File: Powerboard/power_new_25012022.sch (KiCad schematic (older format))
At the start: 25 parts

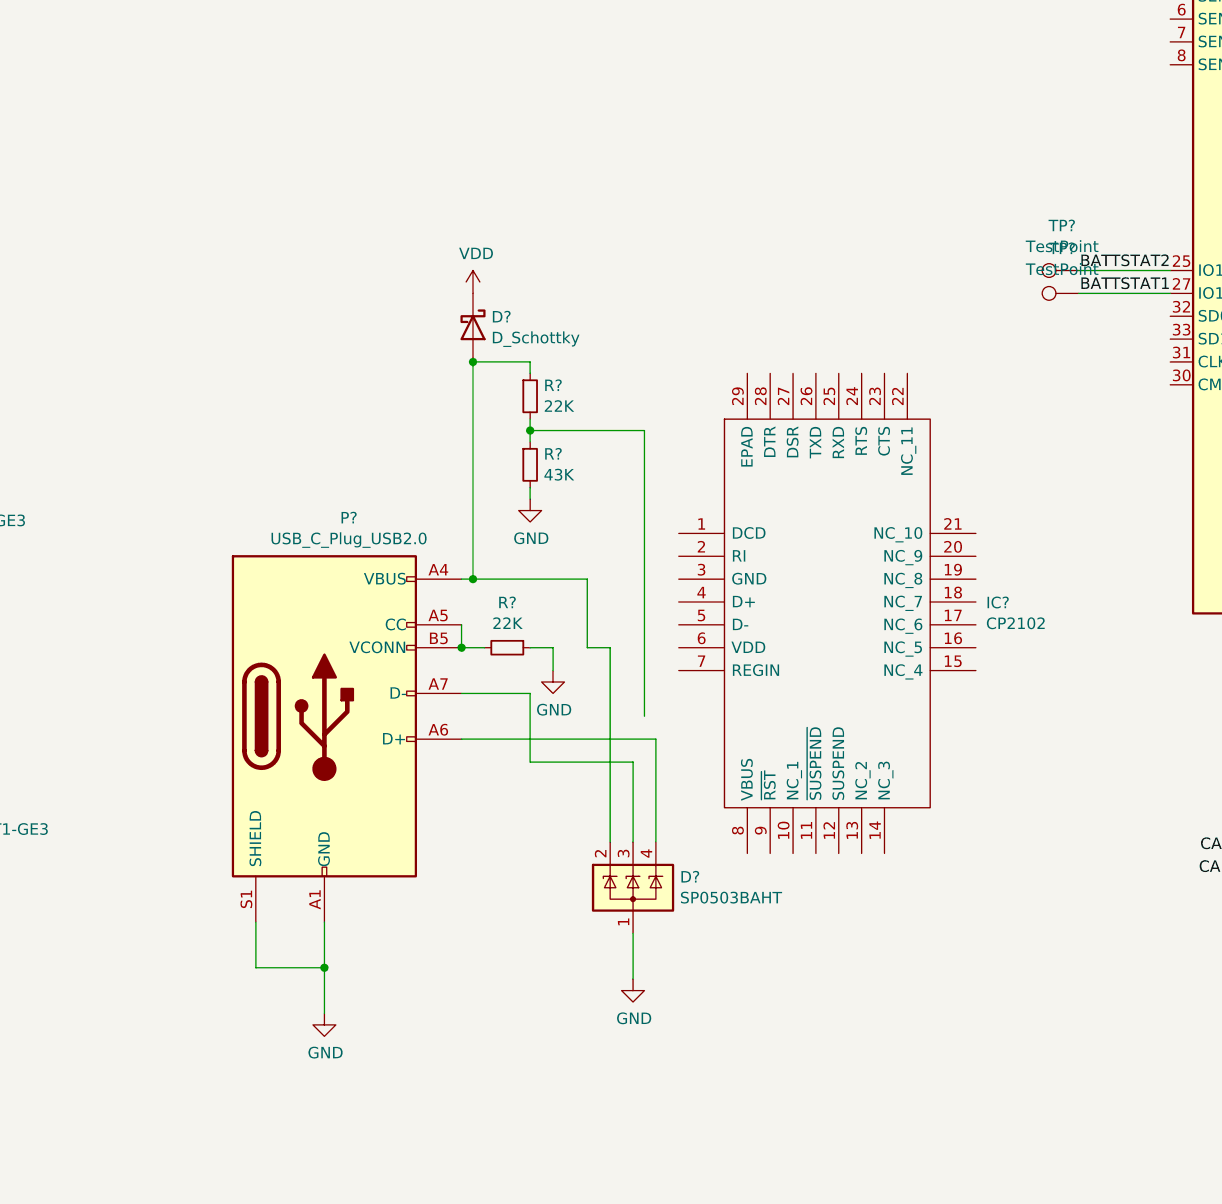
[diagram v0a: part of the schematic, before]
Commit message: 19/02/2022
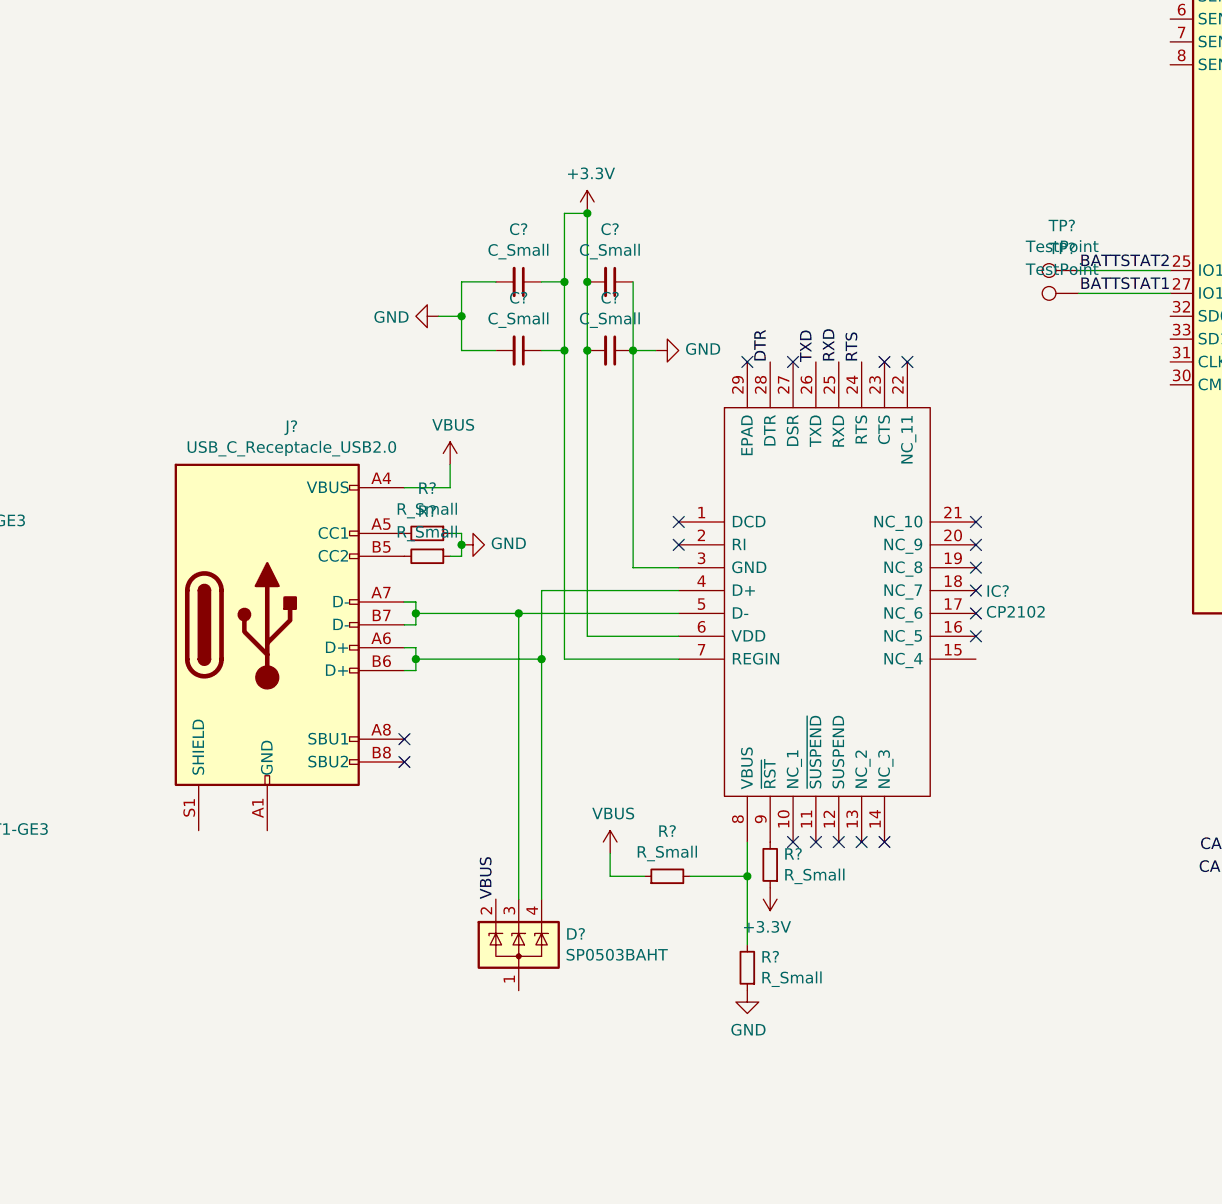
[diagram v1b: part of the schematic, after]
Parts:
- removed D?: SP0503BAHT, Package_TO_SOT_SMD:SOT-143, symbol Power_Protection:SP0503BAHT
- removed D?: D_Schottky, symbol Device:D_Schottky
- removed P?: USB_C_Plug_USB2.0, symbol Connector:USB_C_Plug_USB2.0
- removed R? (x2): 22K, symbol Device:R_Small
- removed R?: 43K, symbol Device:R_Small
- added C? (x4): C_Small, symbol Device:C_Small
- added D?: SP0503BAHT, Package_TO_SOT_SMD:SOT-143, symbol Power_Protection:SP0503BAHT
- added J?: USB_C_Receptacle_USB2.0, symbol Connector:USB_C_Receptacle_USB2.0
- added R? (x5): R_Small, symbol Device:R_Small
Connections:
- net +3V3: now also IC?.6 (VDD), IC?.7 (REGIN), C?.1, C?.1, C?.2, C?.2, R?.1
- net GND: now also IC?.3 (GND), C?.1, C?.1, C?.2, C?.2, R?.1, R?.1, R?.1
- net RXD: now also IC?.25 (RXD)
- net RTS: now reaches IC?.24 (RTS)
- net TXD: now reaches IC?.26 (TXD)
- net DTR: now reaches IC?.28 (DTR)
- net at IC?.4 (D+): now also D?.4 (K), J?.A6 (D+), J?.B6 (D+)
- net at IC?.5 (D-): now also D?.3 (K), J?.A7 (D-), J?.B7 (D-)
- net at IC?.8 (VBUS): now also R?.2, R?.2
- net at IC?.9 (~RST): now also R?.2
- new net: J?.A1 (GND), J?.A12 (GND), J?.B1 (GND), J?.B12 (GND)
- new net: J?.A5 (CC1), R?.2
- new net: J?.B5 (CC2), R?.2
- new net VBUS: D?.2 (K), J?.A4 (VBUS), J?.A9 (VBUS), J?.B4 (VBUS), J?.B9 (VBUS), R?.1
- no-connect marks 2 -> 21
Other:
- moved on the sheet: IC?
